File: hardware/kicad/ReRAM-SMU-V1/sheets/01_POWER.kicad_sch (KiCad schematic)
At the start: 38 parts, among them J1 POWER_IN +-12V EXT 3.5mm pitc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, U1 LT3045EDD +5V_A 500mA 0.8uVrm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, U2 TLV1117-33 +3V3 800mA from +5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, U3 LTC6655BHMS8-5.0 DAC REF 5.0V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, U4 LTC6655BHMS8-2.5 ADC REF 2.5V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, U5 TPS3808G33 supervisor +3V3 Vt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

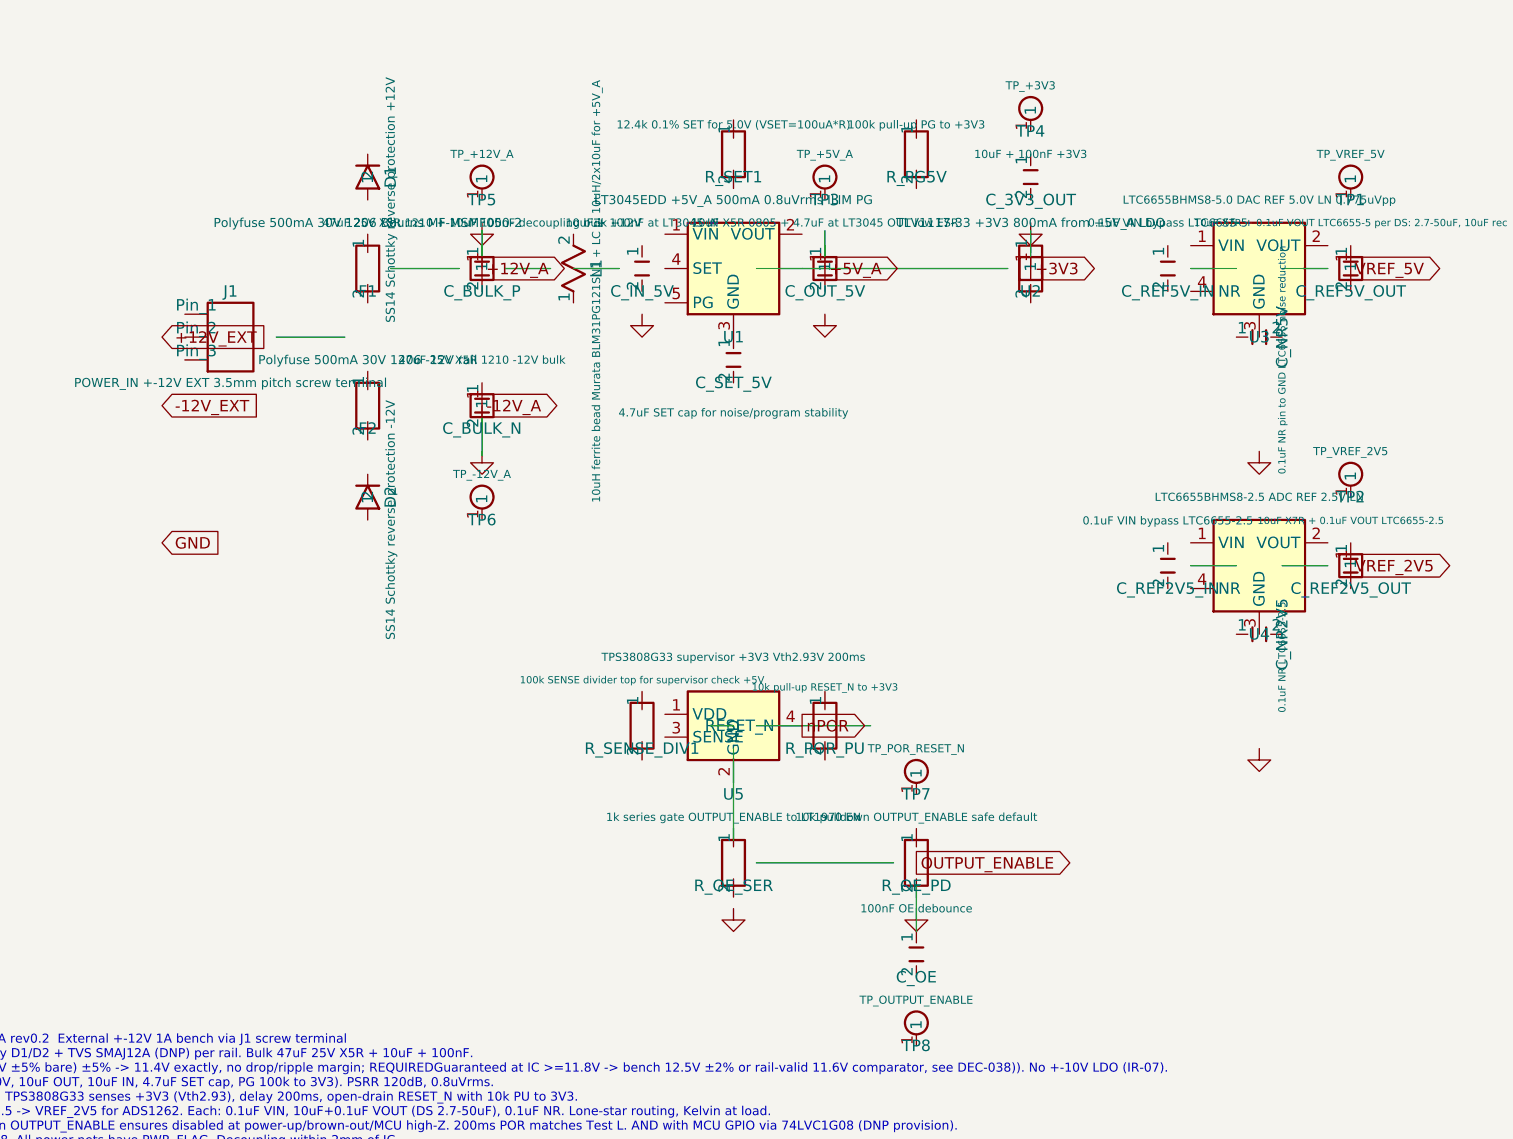
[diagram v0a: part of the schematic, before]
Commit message: Beta
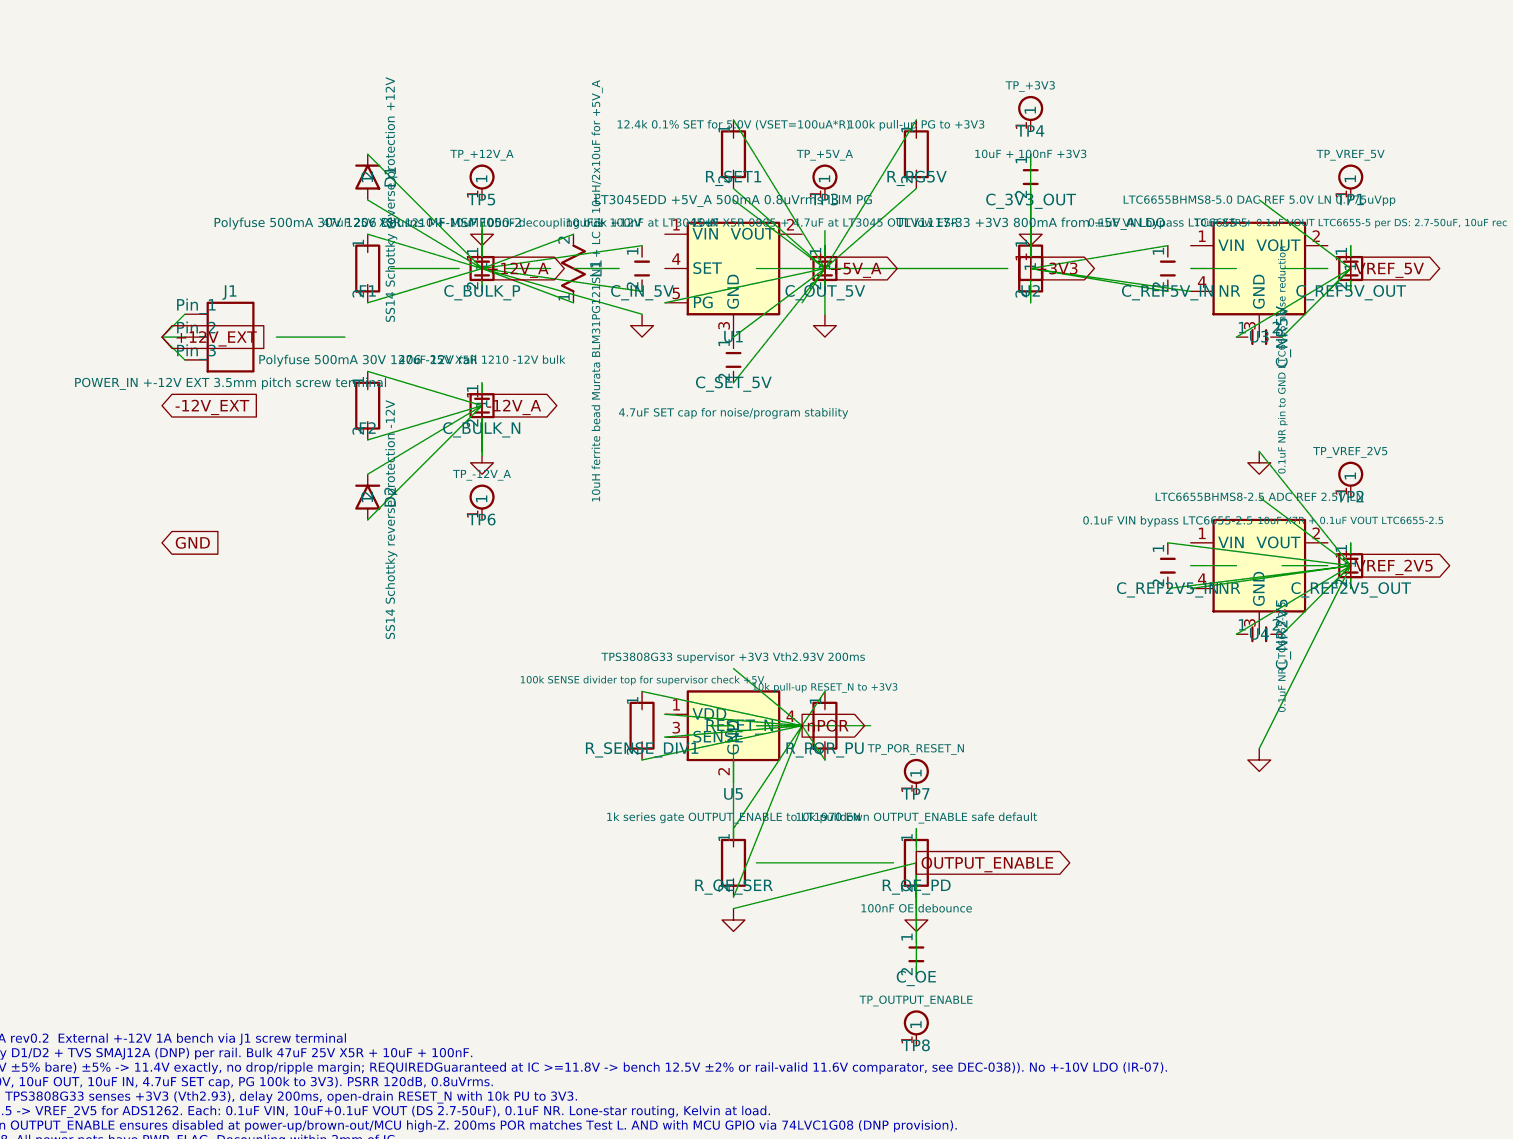
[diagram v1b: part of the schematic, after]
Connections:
- net +12V_A: now also C_BULK_P.1, C_BULK_P.2, C_IN_5V.1, C_IN_5V.2, D1.1, D1.2, F1.1, F1.2, L1.1, L1.2
- net +12V_EXT: now also J1.1 (Pin_1), J1.2 (Pin_2), J1.3 (Pin_3)
- net +3V3: now also C_3V3_OUT.1, C_3V3_OUT.2, C_REF5V_IN.1, C_REF5V_IN.2, U2.1, U2.2, U3.4 (NR)
- net +5V_A: now also C_OUT_5V.1, C_OUT_5V.2, C_SET_5V.1, C_SET_5V.2, R_PG5V.1, R_PG5V.2, R_SET1.1, R_SET1.2, U1.3 (GND), U1.5 (PG)
- net -12V_A: now also C_BULK_N.1, C_BULK_N.2, D2.1, D2.2, F2.1, F2.2
- net OUTPUT_ENABLE: now also C_OE.1, C_OE.2, R_OE_PD.1, R_OE_PD.2
- net VREF_2V5: now also C_NR2V5.1, C_NR2V5.2, C_REF2V5_IN.1, C_REF2V5_IN.2, C_REF2V5_OUT.1, C_REF2V5_OUT.2, U4.4 (NR)
- net VREF_5V: now also C_NR5V.1, C_NR5V.2, C_REF5V_OUT.1, C_REF5V_OUT.2
- net nPOR: now also R_OE_SER.1, R_OE_SER.2, R_POR_PU.1, R_POR_PU.2, R_SENSE_DIV1.1, R_SENSE_DIV1.2, U5.1 (VDD), U5.3 (SENSE)
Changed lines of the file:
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@@
 	(wire (pts (xy 91.44 26.27) (xy 91.44 30.48)) (stroke (width 0) (type default)) (uuid "wire-pwr-correct-91.44-25"))
 	(wire (pts (xy 114.3 26.27) (xy 114.3 30.48)) (stroke (width 0) (type default)) (uuid "wire-pwr-correct-114.3-25"))
+	(wire (pts (xy 20.320 40.640) (xy 17.780 38.100)) (stroke (width 0) (type default)))
+	(wire (pts (xy 20.320 38.100) (xy 17.780 38.100)) (stroke (width 0) (type default)))
+	(wire (pts (xy 20.320 35.560) (xy 17.780 38.100)) (stroke (width 0) (type default)))
+	(wire (pts (xy 40.640 34.290) (xy 53.340 30.480)) (stroke (width 0) (type default)))
+	(wire (pts (xy 40.640 26.670) (xy 53.340 30.480)) (stroke (width 0) (type default)))
+	(wire (pts (xy 40.640 49.530) (xy 53.340 45.720)) (stroke (width 0) (type default)))
+	(wire (pts (xy 40.640 41.910) (xy 53.340 45.720)) (stroke (width 0) (type default)))
+	(wire (pts (xy 40.640 17.780) (xy 53.340 30.480)) (stroke (width 0) (type default)))
+	(wire (pts (xy 40.640 22.860) (xy 53.340 30.480)) (stroke (width 0) (type default)))
+	(wire (pts (xy 40.640 53.340) (xy 53.340 45.720)) (stroke (width 0) (type default)))
+	(wire (pts (xy 40.640 58.420) (xy 53.340 45.720)) (stroke (width 0) (type default)))
+	(wire (pts (xy 53.340 33.020) (xy 53.340 30.480)) (stroke (width 0) (type default)))
+	(wire (pts (xy 53.340 27.940) (xy 53.340 30.480)) (stroke (width 0) (type default)))
+	(wire (pts (xy 53.340 48.260) (xy 53.340 45.720)) (stroke (width 0) (type default)))
+	(wire (pts (xy 53.340 43.180) (xy 53.340 45.720)) (stroke (width 0) (type default)))
+	(wire (pts (xy 63.500 26.670) (xy 53.340 30.480)) (stroke (width 0) (type default)))
+	(wire (pts (xy 63.500 34.290) (xy 53.340 30.480)) (stroke (width 0) (type default)))
+	(wire (pts (xy 73.660 34.290) (xy 91.440 30.480)) (stroke (width 0) (type default)))
+	(wire (pts (xy 88.900 34.290) (xy 91.440 30.480)) (stroke (width 0) (type default)))
+	(wire (pts (xy 81.280 22.860) (xy 91.440 30.480)) (stroke (width 0) (type default)))
+	(wire (pts (xy 81.280 21.590) (xy 91.440 30.480)) (stroke (width 0) (type default)))
+	(wire (pts (xy 81.280 13.970) (xy 91.440 30.480)) (stroke (width 0) (type default)))
+	(wire (pts (xy 91.440 33.020) (xy 91.440 30.480)) (stroke (width 0) (type default)))
+	(wire (pts (xy 91.440 27.940) (xy 91.440 30.480)) (stroke (width 0) (type default)))
+	(wire (pts (xy 71.120 33.020) (xy 53.340 30.480)) (stroke (width 0) (type default)))
+	(wire (pts (xy 71.120 27.940) (xy 53.340 30.480)) (stroke (width 0) (type default)))
+	(wire (pts (xy 101.600 21.590) (xy 91.440 30.480)) (stroke (width 0) (type default)))
+	(wire (pts (xy 101.600 13.970) (xy 91.440 30.480)) (stroke (width 0) (type default)))
+	(wire (pts (xy 81.280 43.180) (xy 91.440 30.480)) (stroke (width 0) (type default)))
+	(wire (pts (xy 81.280 38.100) (xy 91.440 30.480)) (stroke (width 0) (type default)))
+	(wire (pts (xy 114.300 34.290) (xy 114.300 30.480)) (stroke (width 0) (type default)))
+	(wire (pts (xy 114.300 26.670) (xy 114.300 30.480)) (stroke (width 0) (type default)))
+	(wire (pts (xy 114.300 22.860) (xy 114.300 30.480)) (stroke (width 0) (type default)))
+	(wire (pts (xy 114.300 17.780) (xy 114.300 30.480)) (stroke (width 0) (type default)))
+	(wire (pts (xy 132.080 33.020) (xy 114.300 30.480)) (stroke (width 0) (type default)))
+	(wire (pts (xy 147.320 33.020) (xy 149.860 30.480)) (stroke (width 0) (type default)))
+	(wire (pts (xy 139.700 22.860) (xy 149.860 30.480)) (stroke (width 0) (type default)))
+	(wire (pts (xy 129.540 33.020) (xy 114.300 30.480)) (stroke (width 0) (type default)))
+	(wire (pts (xy 129.540 27.940) (xy 114.300 30.480)) (stroke (width 0) (type default)))
+	(wire (pts (xy 149.860 33.020) (xy 149.860 30.480)) (stroke (width 0) (type default)))
+	(wire (pts (xy 149.860 27.940) (xy 149.860 30.480)) (stroke (width 0) (type default)))
+	(wire (pts (xy 137.160 38.100) (xy 149.860 30.480)) (stroke (width 0) (type default)))
+	(wire (pts (xy 142.240 38.100) (xy 149.860 30.480)) (stroke (width 0) (type default)))
+	(wire (pts (xy 132.080 66.040) (xy 149.860 63.500)) (stroke (width 0) (type default)))
+	(wire (pts (xy 147.320 66.040) (xy 149.860 63.500)) (stroke (width 0) (type default)))
+	(wire (pts (xy 139.700 55.880) (xy 149.860 63.500)) (stroke (width 0) (type default)))
+	(wire (pts (xy 129.540 66.040) (xy 149.860 63.500)) (stroke (width 0) (type default)))
+	(wire (pts (xy 129.540 60.960) (xy 149.860 63.500)) (stroke (width 0) (type default)))
+	(wire (pts (xy 149.860 66.040) (xy 149.860 63.500)) (stroke (width 0) (type default)))
+	(wire (pts (xy 149.860 60.960) (xy 149.860 63.500)) (stroke (width 0) (type default)))
+	(wire (pts (xy 137.160 71.120) (xy 149.860 63.500)) (stroke (width 0) (type default)))
+	(wire (pts (xy 142.240 71.120) (xy 149.860 63.500)) (stroke (width 0) (type default)))
+	(wire (pts (xy 73.660 82.550) (xy 88.900 81.280)) (stroke (width 0) (type default)))
+	(wire (pts (xy 81.280 74.930) (xy 88.900 81.280)) (stroke (width 0) (type default)))
+	(wire (pts (xy 73.660 80.010) (xy 88.900 81.280)) (stroke (width 0) (type default)))
+	(wire (pts (xy 71.120 85.090) (xy 88.900 81.280)) (stroke (width 0) (type default)))
+	(wire (pts (xy 71.120 77.470) (xy 88.900 81.280)) (stroke (width 0) (type default)))
+	(wire (pts (xy 91.440 85.090) (xy 88.900 81.280)) (stroke (width 0) (type default)))
+	(wire (pts (xy 91.440 77.470) (xy 88.900 81.280)) (stroke (width 0) (type default)))
+	(wire (pts (xy 101.600 100.330) (xy 101.600 96.520)) (stroke (width 0) (type default)))
+	(wire (pts (xy 101.600 92.710) (xy 101.600 96.520)) (stroke (width 0) (type default)))
+	(wire (pts (xy 81.280 100.330) (xy 88.900 81.280)) (stroke (width 0) (type default)))
+	(wire (pts (xy 81.280 92.710) (xy 88.900 81.280)) (stroke (width 0) (type default)))
+	(wire (pts (xy 101.600 109.220) (xy 101.600 96.520)) (stroke (width 0) (type default)))
+	(wire (pts (xy 53.340 31.750) (xy 53.340 30.480)) (stroke (width 0) (type default)))
+	(wire (pts (xy 53.340 46.990) (xy 53.340 45.720)) (stroke (width 0) (type default)))
+	(wire (pts (xy 91.440 31.750) (xy 91.440 30.480)) (stroke (width 0) (type default)))
+	(wire (pts (xy 114.300 31.750) (xy 114.300 30.480)) (stroke (width 0) (type default)))
+	(wire (pts (xy 149.860 31.750) (xy 149.860 30.480)) (stroke (width 0) (type default)))
+	(wire (pts (xy 149.860 64.770) (xy 149.860 63.500)) (stroke (width 0) (type default)))
+	(wire (pts (xy 71.120 35.560) (xy 53.340 30.480)) (stroke (width 0) (type default)))
+	(wire (pts (xy 91.440 35.560) (xy 91.440 30.480)) (stroke (width 0) (type default)))
+	(wire (pts (xy 114.300 25.400) (xy 114.300 30.480)) (stroke (width 0) (type default)))
+	(wire (pts (xy 139.700 50.800) (xy 149.860 63.500)) (stroke (width 0) (type default)))
+	(wire (pts (xy 139.700 83.820) (xy 149.860 63.500)) (stroke (width 0) (type default)))
+	(wire (pts (xy 81.280 101.600) (xy 101.600 96.520)) (stroke (width 0) (type default)))
+	(wire (pts (xy 101.600 101.600) (xy 101.600 96.520)) (stroke (width 0) (type default)))
+	(wire (pts (xy 53.340 25.400) (xy 53.340 30.480)) (stroke (width 0) (type default)))
+	(wire (pts (xy 53.340 50.800) (xy 53.340 45.720)) (stroke (width 0) (type default)))
 )
